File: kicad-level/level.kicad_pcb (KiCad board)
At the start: 2 copper layers, 62.9 x 27.4 mm, 6 parts, among them J1 Conn_01x01_Pin, J2 Conn_01x08_Pin, J3 Conn_01x01_Pin, U1 ULN2803A_C845537

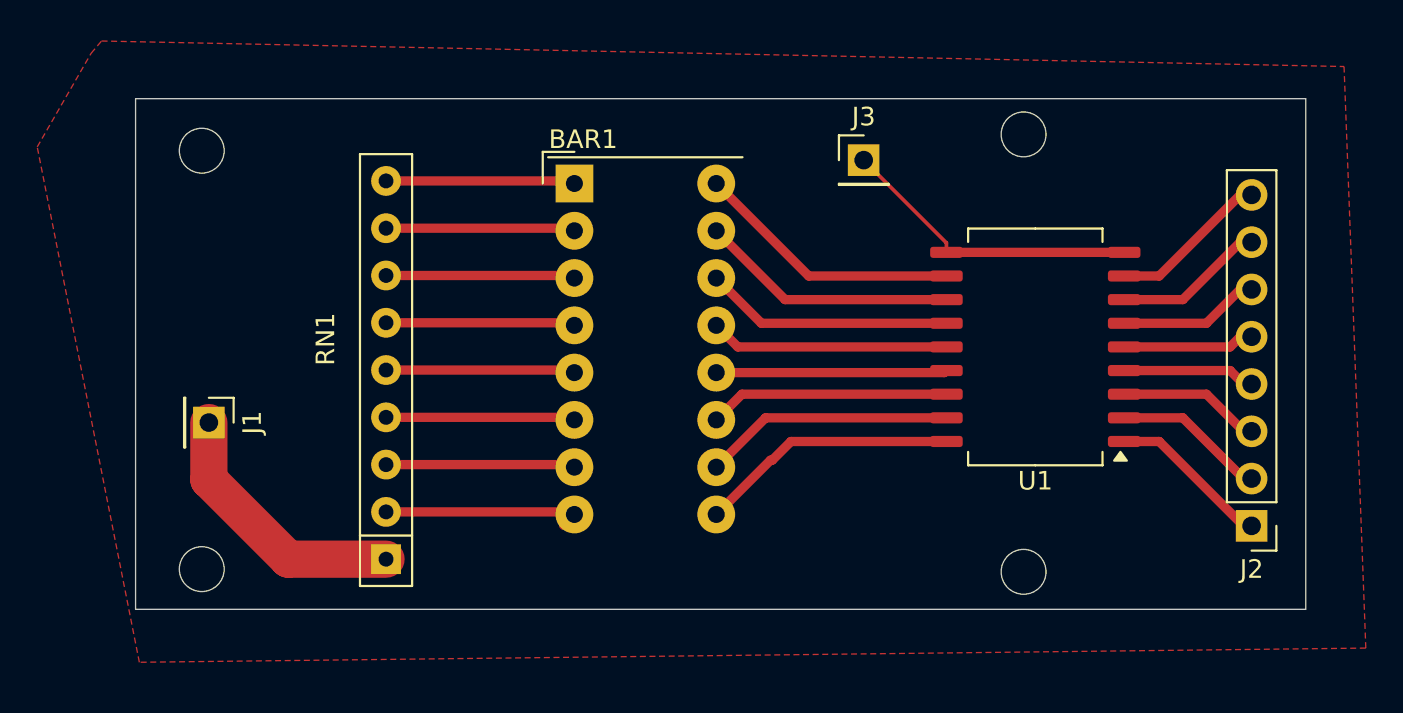
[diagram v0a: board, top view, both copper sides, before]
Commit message: misa a jour pcb plus petit
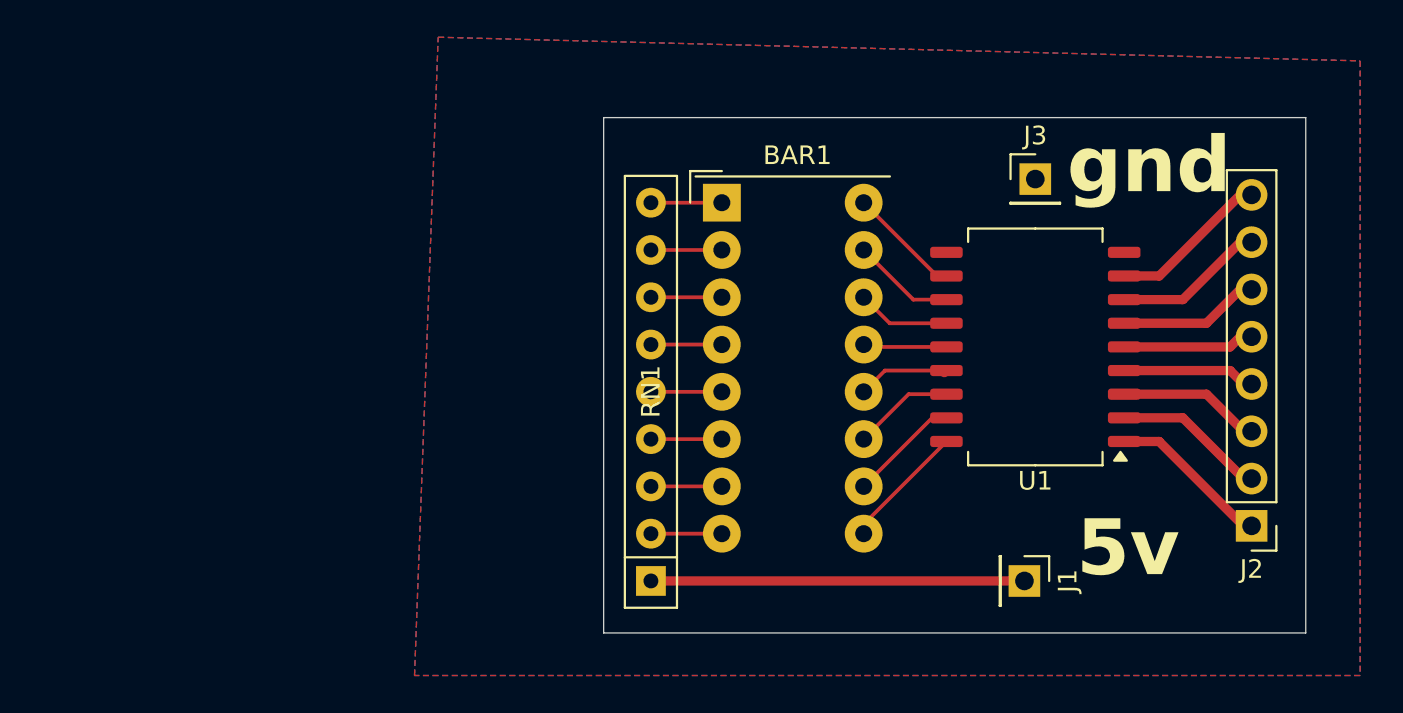
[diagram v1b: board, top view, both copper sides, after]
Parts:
- moved J1 44.6 mm to (177.5, 110.5)
- moved RN1 14.3 mm to (157.5, 110.5)
- moved J3 9.28 mm to (178.1, 88.9)
- moved BAR1 7.99 mm to (161.3, 90.2)
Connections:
- U1 pad 10: GND -> unconnected-(U1-COM-Pad10)
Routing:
- net GND: track 16.3 -> 0.00 mm
- net Net-(U1-O5): track 12.8 -> 4.50 mm
- net Net-(U1-O8): track 14.4 -> 6.08 mm
- net Net-(U1-O7): track 13.9 -> 5.55 mm
- net Net-(U1-O6): track 13.4 -> 5.02 mm
- net Net-(U1-O2): track 13.5 -> 5.97 mm
- net Net-(U1-O3): track 12.9 -> 5.44 mm
- net Net-(U1-O4): track 12.4 -> 5.08 mm
- net Net-(U1-O1): track 14.0 -> 6.79 mm
- net Net-(RN1-R1): track 11.0 -> 3.81 mm
- net Net-(RN1-R3): track 10.7 -> 3.81 mm
- net Net-(RN1-R8): track 10.2 -> 3.81 mm
- net Net-(RN1-R6): track 10.2 -> 3.81 mm
- net Net-(RN1-R4): track 10.2 -> 3.81 mm
- net Net-(RN1-R2): track 10.2 -> 3.81 mm
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- added copper zone on B.Cu, net GND
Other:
- board size 62.9 x 27.4 mm -> 37.7 x 27.7 mm
- board text added: "5v"
- board text added: "gnd"
